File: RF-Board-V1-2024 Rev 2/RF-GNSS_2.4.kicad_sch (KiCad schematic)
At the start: 33 parts, among them J4 UART, J5 RFPC-SMA28-F, J6 RFPC-SMA29-F, SW4 SW_SPST, SW5 SW_SPST

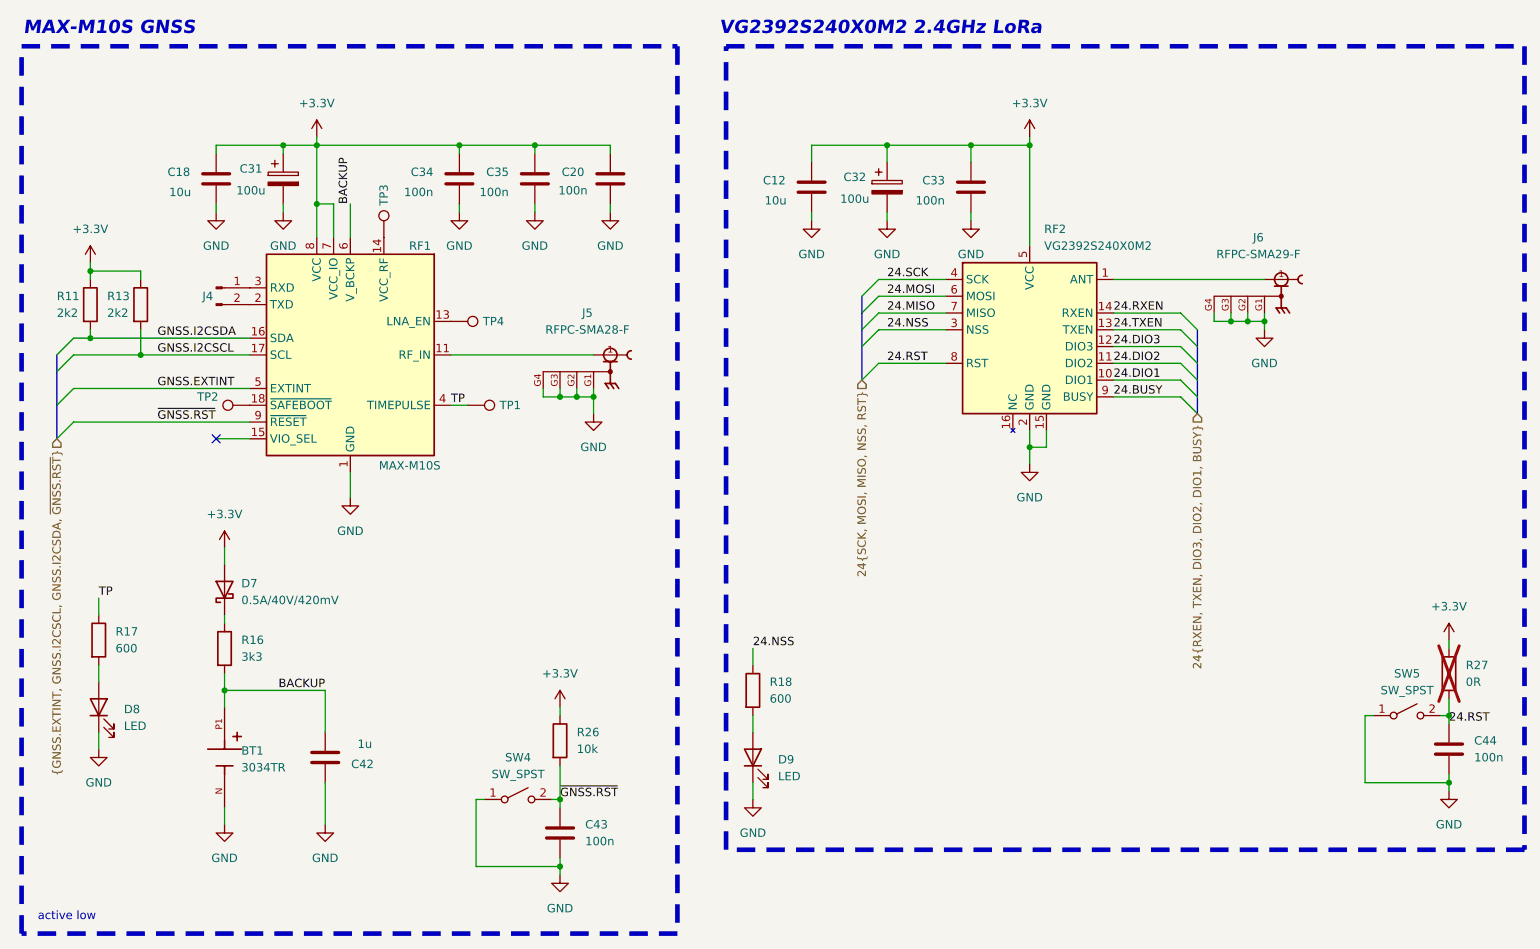
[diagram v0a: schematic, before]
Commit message: made some notes
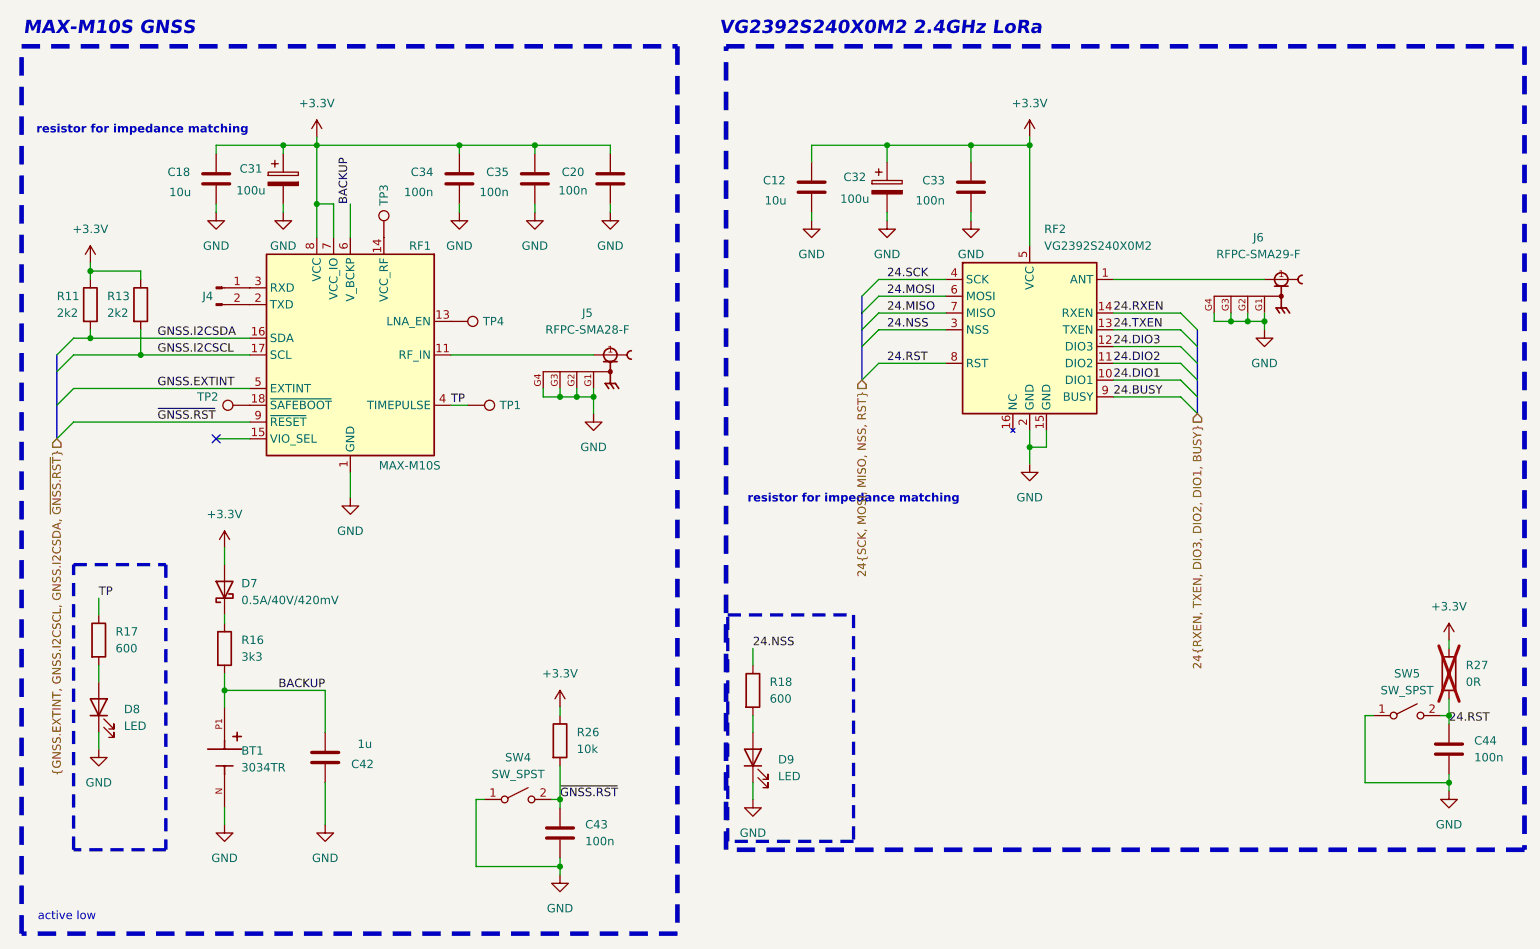
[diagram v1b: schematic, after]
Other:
- note added: "resistor for impedance matching"
